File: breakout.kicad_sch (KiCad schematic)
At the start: 9 parts, among them J2 Conn_01x09_Socket, U4 HV5622PG, U5 HV5622PG

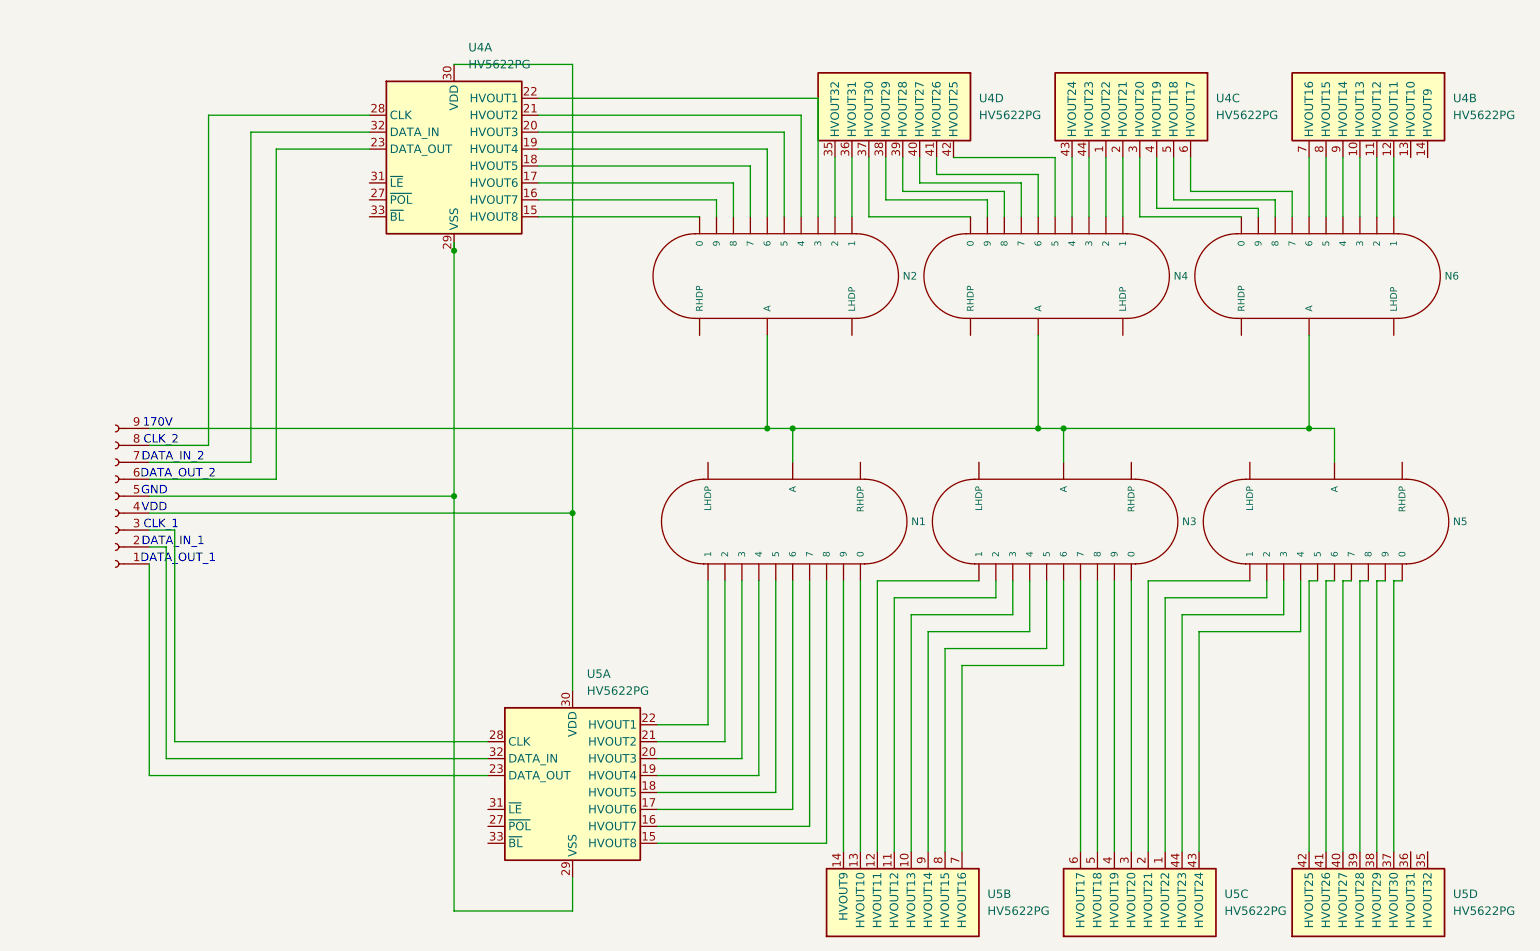
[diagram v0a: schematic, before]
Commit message: ywah
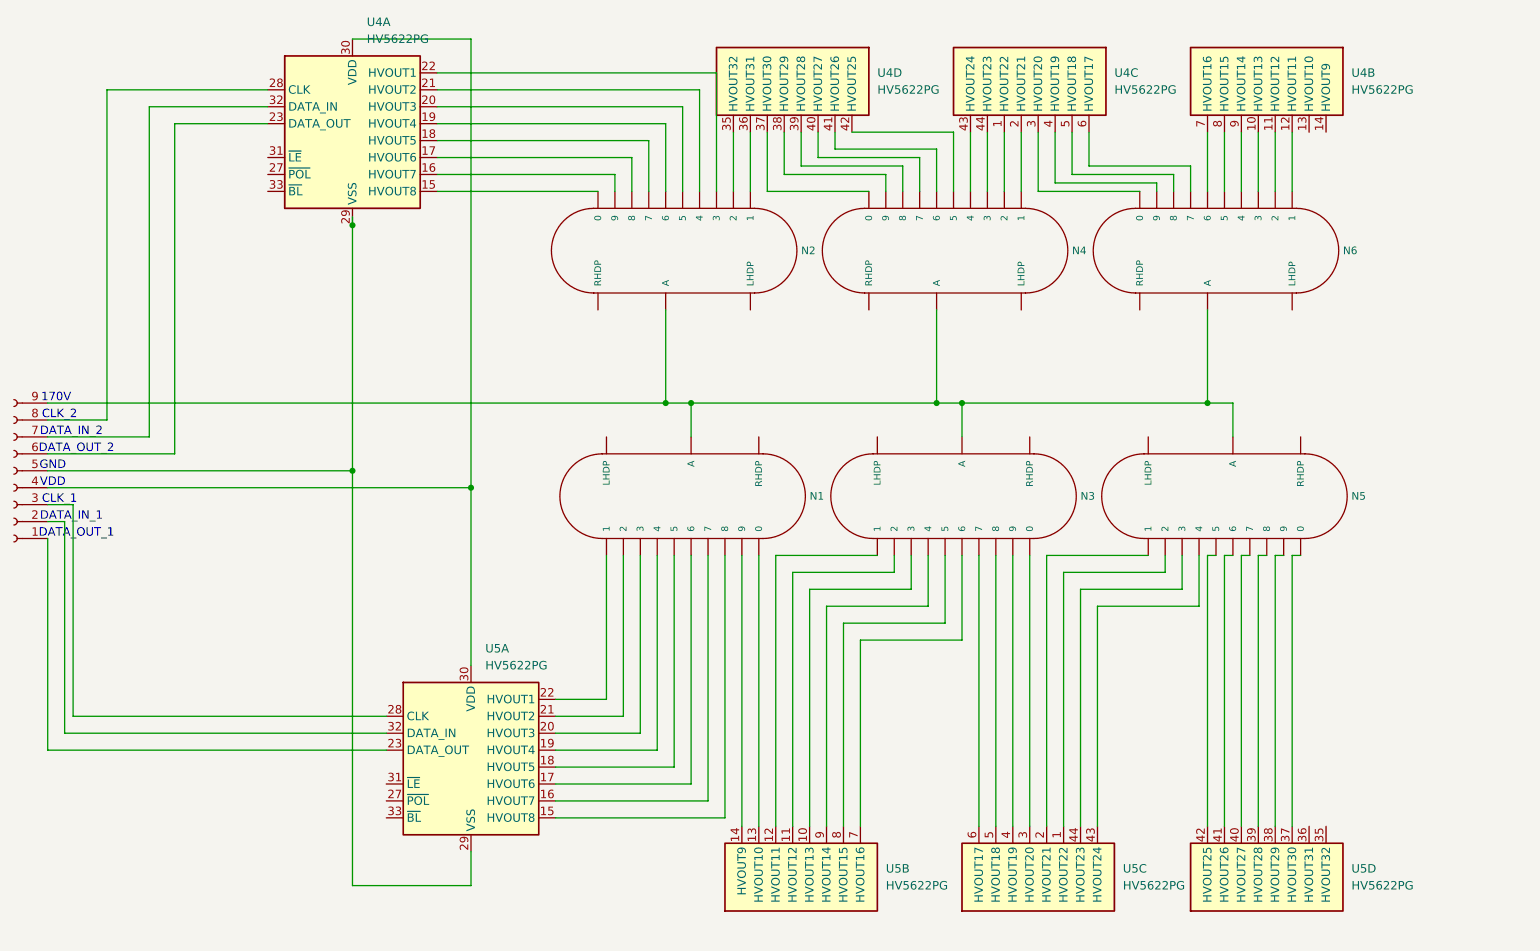
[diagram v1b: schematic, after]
